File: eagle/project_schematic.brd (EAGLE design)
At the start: 60.9 x 59.4 mm, 17 parts, among them Q1 2N3904, Q2 2N3904, Q3 2N3906

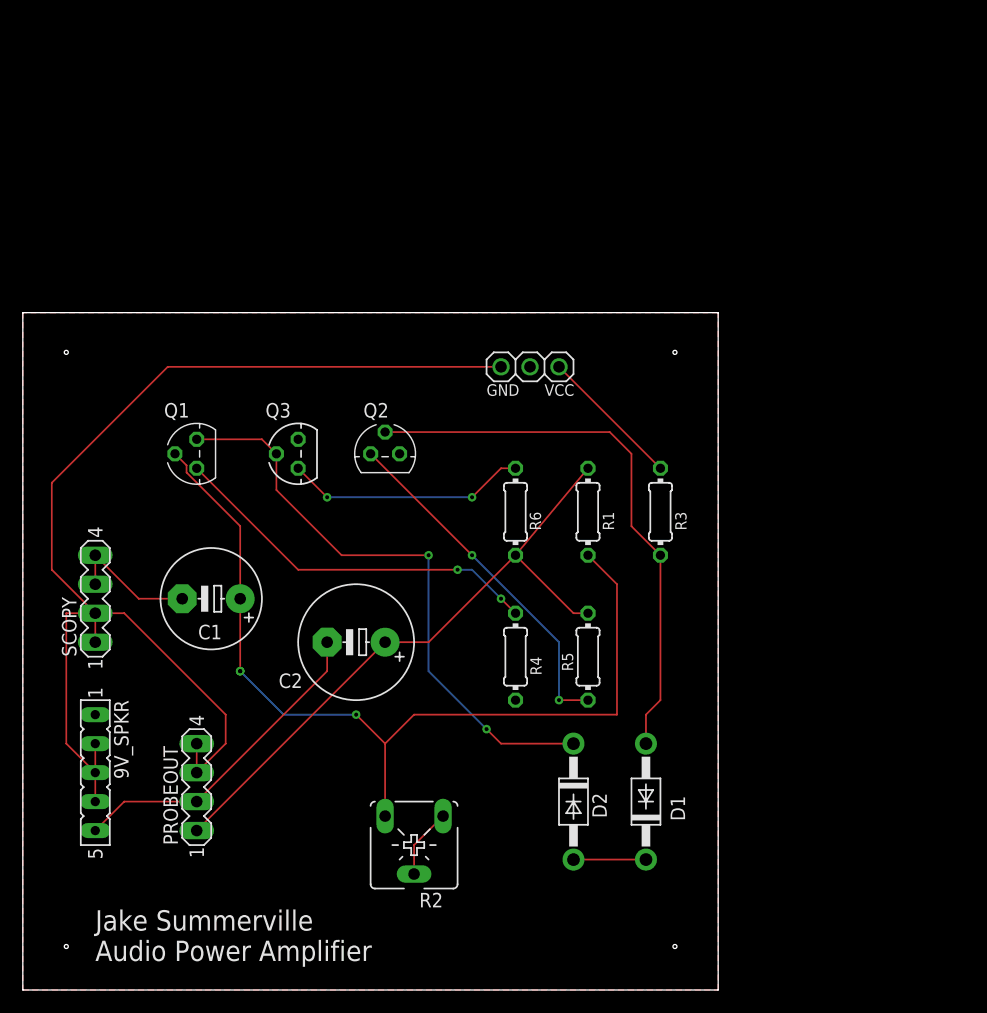
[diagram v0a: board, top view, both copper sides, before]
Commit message: Increased size
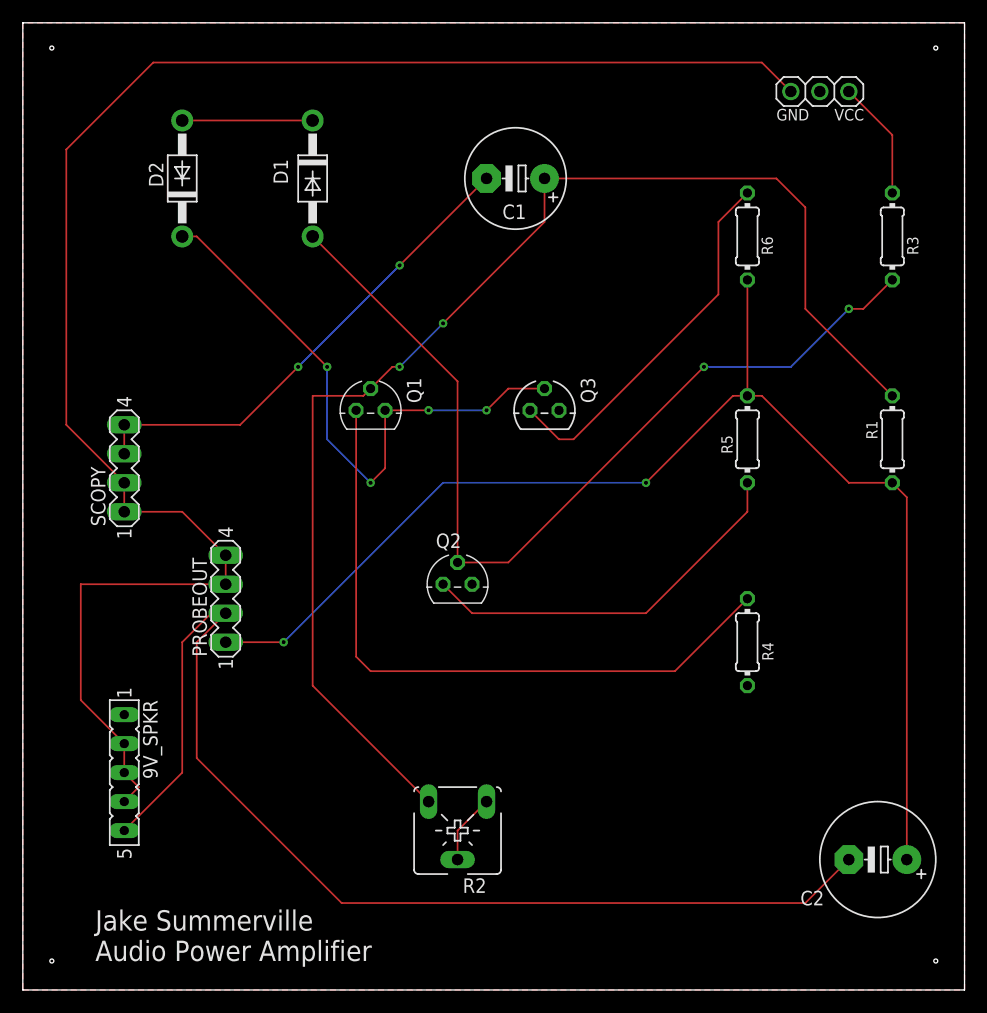
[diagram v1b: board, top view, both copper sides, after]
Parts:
- moved D2 64.5 mm to (14.0, 71.1), turned to 90 degrees
- moved D1 61.9 mm to (25.4, 71.1), turned to 270 degrees
- moved C2 49.5 mm to (74.9, 11.4)
- moved C1 45.5 mm to (43.2, 71.1)
- moved POWER 35.0 mm to (69.8, 78.7)
- moved R3 31.5 mm to (76.2, 66.0)
- moved R6 31.5 mm to (63.5, 66.0)
- moved R1 27.4 mm to (76.2, 48.3), turned to 90 degrees
- moved R5 23.6 mm to (63.5, 48.3)
- moved Q3 21.9 mm to (45.7, 50.8), turned to 0 degrees
- moved R4 20.4 mm to (63.5, 30.5)
- moved PROBEOUT 16.7 mm to (17.8, 34.3)
- moved Q1 15.7 mm to (30.5, 50.8), turned to 0 degrees
- moved Q2 13.1 mm to (38.1, 35.6)
- moved SCOPY 11.7 mm to (8.89, 45.7)
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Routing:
- net N$11: track 28.6 -> 101.2 mm
- net VN: track 56.3 -> 114.2 mm, vias 0 -> 2
- net GND: track 105.6 -> 149.0 mm
- net N$1: track 79.5 -> 113.8 mm, vias 3 -> 2
- net N$5: track 49.4 -> 82.2 mm, vias 0 -> 2
- net N$17: track 11.7 -> 43.2 mm, vias 0 -> 2
- net N$2: track 33.2 -> 59.0 mm, vias 2 -> 0
- net N$10: track 21.2 -> 32.8 mm, vias 2 -> 0
- net N$8: track 6.35 -> 11.4 mm
- net N$9: track 31.0 -> 33.9 mm, vias 2 -> 0
- net VCC: track 12.6 -> 10.5 mm
- net N$3: track 51.9 -> 50.8 mm, vias 2 -> 4
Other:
- board size 60.9 x 59.4 mm -> 82.5 x 84.8 mm
